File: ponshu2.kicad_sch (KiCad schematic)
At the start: 0 parts

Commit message: create sch file
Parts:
- added U1: STM32F072CBTx, Package_QFP:LQFP-48_7x7mm_P0.5mm, symbol MCU_ST_STM32F0:STM32F072CBTx
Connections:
- new net: U1.23 (VSS), U1.35 (VSS), U1.47 (VSS)
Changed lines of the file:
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@@
 	(generator_version "9.0")
 	(paper "A4")
+	(symbol
+		(lib_id "MCU_ST_STM32F0:STM32F072CBTx")
+		(at 114.3 82.55 0)
+		(unit 1)
+		(exclude_from_sim no)
+		(in_bom yes)
+		(on_board yes)
+		(dnp no)
+		(fields_autoplaced yes)
+		(property "Reference" "U1"
+			(at 118.9833 123.19 0)
+			(effects
+				(font
+					(size 1.27 1.27)
+				)
+				(justify left)
+			)
+		)
+		(property "Value" "STM32F072CBTx"
+			(at 118.9833 125.73 0)
+			(effects
+				(font
+					(size 1.27 1.27)
+				)
+				(justify left)
+			)
+		)
+		(property "Footprint" "Package_QFP:LQFP-48_7x7mm_P0.5mm"
+			(at 99.06 120.65 0)
+			(effects
+				(font
+					(size 1.27 1.27)
+				)
+				(justify right)
+				(hide yes)
+			)
+		)
+		(property "Datasheet" "https://www.st.com/resource/en/datasheet/stm32f072cb.pdf"
+			(at 114.3 82.55 0)
+			(effects
+				(font
+					(size 1.27 1.27)
+				)
+				(hide yes)
+			)
+		)
+		(property "Description" "STMicroelectronics Arm Cortex-M0 MCU, 128KB flash, 16KB RAM, 48 MHz, 2.0-3.6V, 37 GPIO, LQFP48"
+			(at 114.3 82.55 0)
+			(effects
+				(font
+					(size 1.27 1.27)
+				)
+				(hide yes)
+			)
+		)
+		(pin "12"
+		)
+		(pin "13"
+		)
+		(pin "14"
+		)
+		(pin "15"
+		)
+		(pin "16"
+		)
+		(pin "2"
+		)
+		(pin "3"
+		)
+		(pin "4"
+		)
+		(pin "18"
+		)
+		(pin "39"
+		)
+		(pin "40"
+		)
+		(pin "41"
+		)
+		(pin "42"
+		)
+		(pin "43"
+		)
+		(pin "45"
+		)
+		(pin "46"
+		)
+		(pin "21"
+		)
+		(pin "22"
+		)
+		(pin "25"
+		)
+		(pin "26"
+		)
+		(pin "27"
+		)
+		(pin "28"
+		)
+		(pin "1"
+		)
+		(pin "24"
+		)
+		(pin "48"
+		)
+		(pin "23"
+		)
+		(pin "35"
+		)
+		(pin "47"
+		)
+		(pin "9"
+		)
+		(pin "8"
+		)
+		(pin "36"
+		)
+		(pin "5"
+		)
+		(pin "19"
+		)
+		(pin "20"
+		)
+		(pin "10"
+		)
+		(pin "11"
+		)
+		(pin "34"
+		)
+		(pin "37"
+		)
+		(pin "38"
+		)
+		(pin "17"
+		)
+		(pin "29"
+		)
+		(pin "30"
+		)
+		(pin "31"
+		)
+		(pin "32"
+		)
+		(pin "33"
+		)
+		(pin "6"
+		)
+		(pin "44"
+		)
+		(pin "7"
+		)
+		(instances
+			(project ""
+				(path "/9a6ee9bd-87da-4626-8a0a-46205075074e"
+					(reference "U1")
+					(unit 1)
+				)
+			)
+		)
+	)
 	(sheet_instances
 		(path "/"

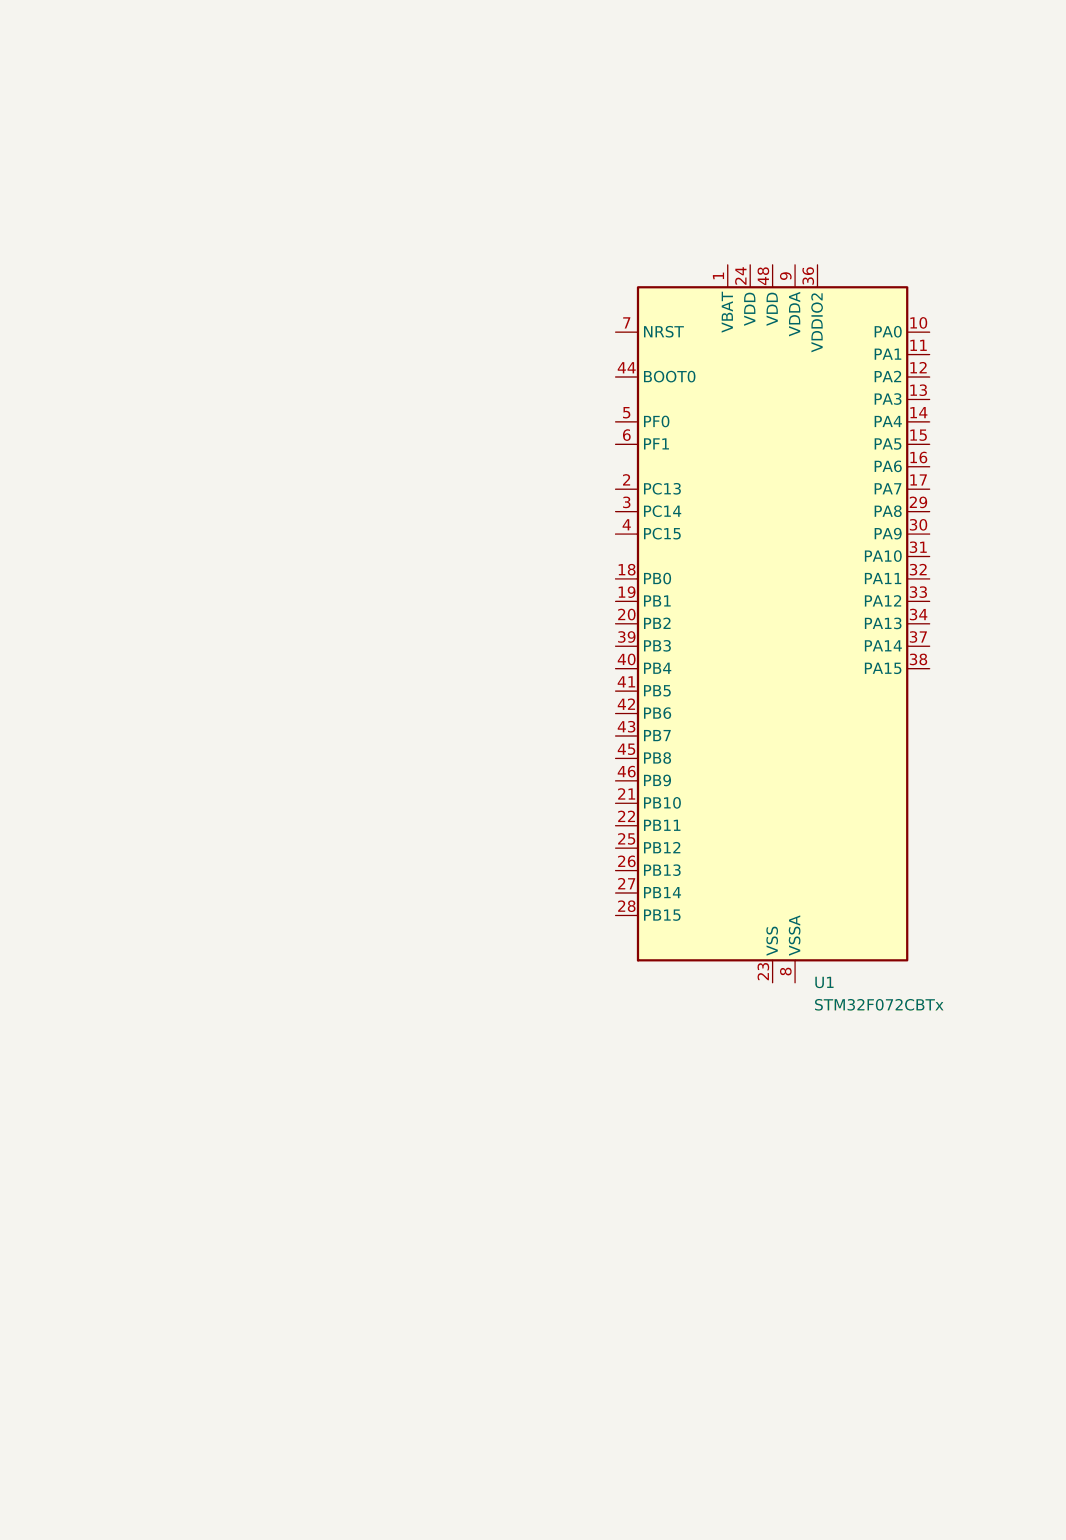
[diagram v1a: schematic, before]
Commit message: chotto PCB tukutayo
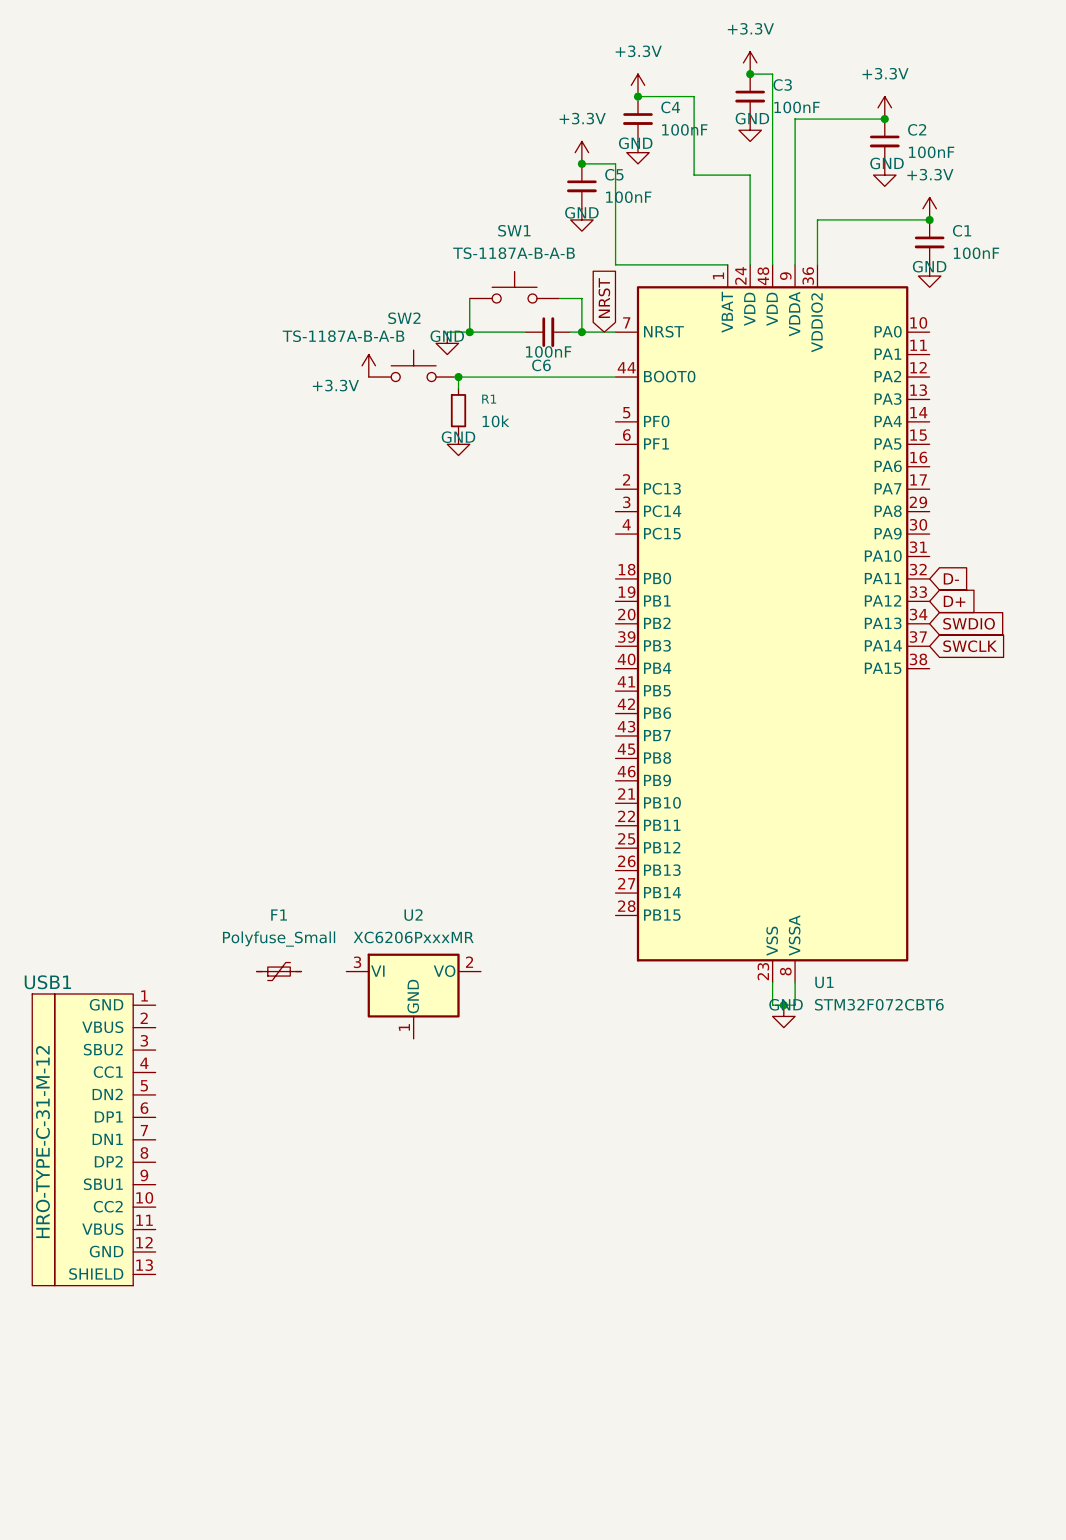
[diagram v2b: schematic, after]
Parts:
- added C1, C2, C3, C4, C5, C6: 100nF, symbol Device:C_Small
- added F1: Polyfuse_Small, symbol Device:Polyfuse_Small
- added R1: 10k, symbol Device:R_Small
- added SW1, SW2: TS-1187A-B-A-B, symbol Switch:SW_Push
- added U2: XC6206PxxxMR, Package_TO_SOT_SMD:SOT-23-3, symbol Regulator_Linear:XC6206PxxxMR
- added USB1: HRO-TYPE-C-31-M-12, symbol Type-C:HRO-TYPE-C-31-M-12
- U1: value STM32F072CBTx -> STM32F072CBT6
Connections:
- net +3.3V: now reaches U1.1 (VBAT)
- net +3.3V: now also U1.24 (VDD), U1.36 (VDDIO2), U1.48 (VDD), U1.9 (VDDA), C1.1, C2.1, C3.1, C4.1, C5.1, SW2.1
- net GND: now reaches U1.23 (VSS), U1.35 (VSS), U1.47 (VSS)
- net GND: now also U1.8 (VSSA), C1.2, C2.2, C3.2, C4.2, C5.2, C6.1, R1.2, SW1.1
- net D-: now reaches U1.32 (PA11)
- net D+: now reaches U1.33 (PA12)
- net SWDIO: now reaches U1.34 (PA13)
- net SWCLK: now reaches U1.37 (PA14)
- net at U1.44 (BOOT0): now also R1.1, SW2.2
- net NRST: now reaches U1.7 (NRST)
- net NRST: now also C6.2, SW1.2

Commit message: PCB daitai owatta kamo
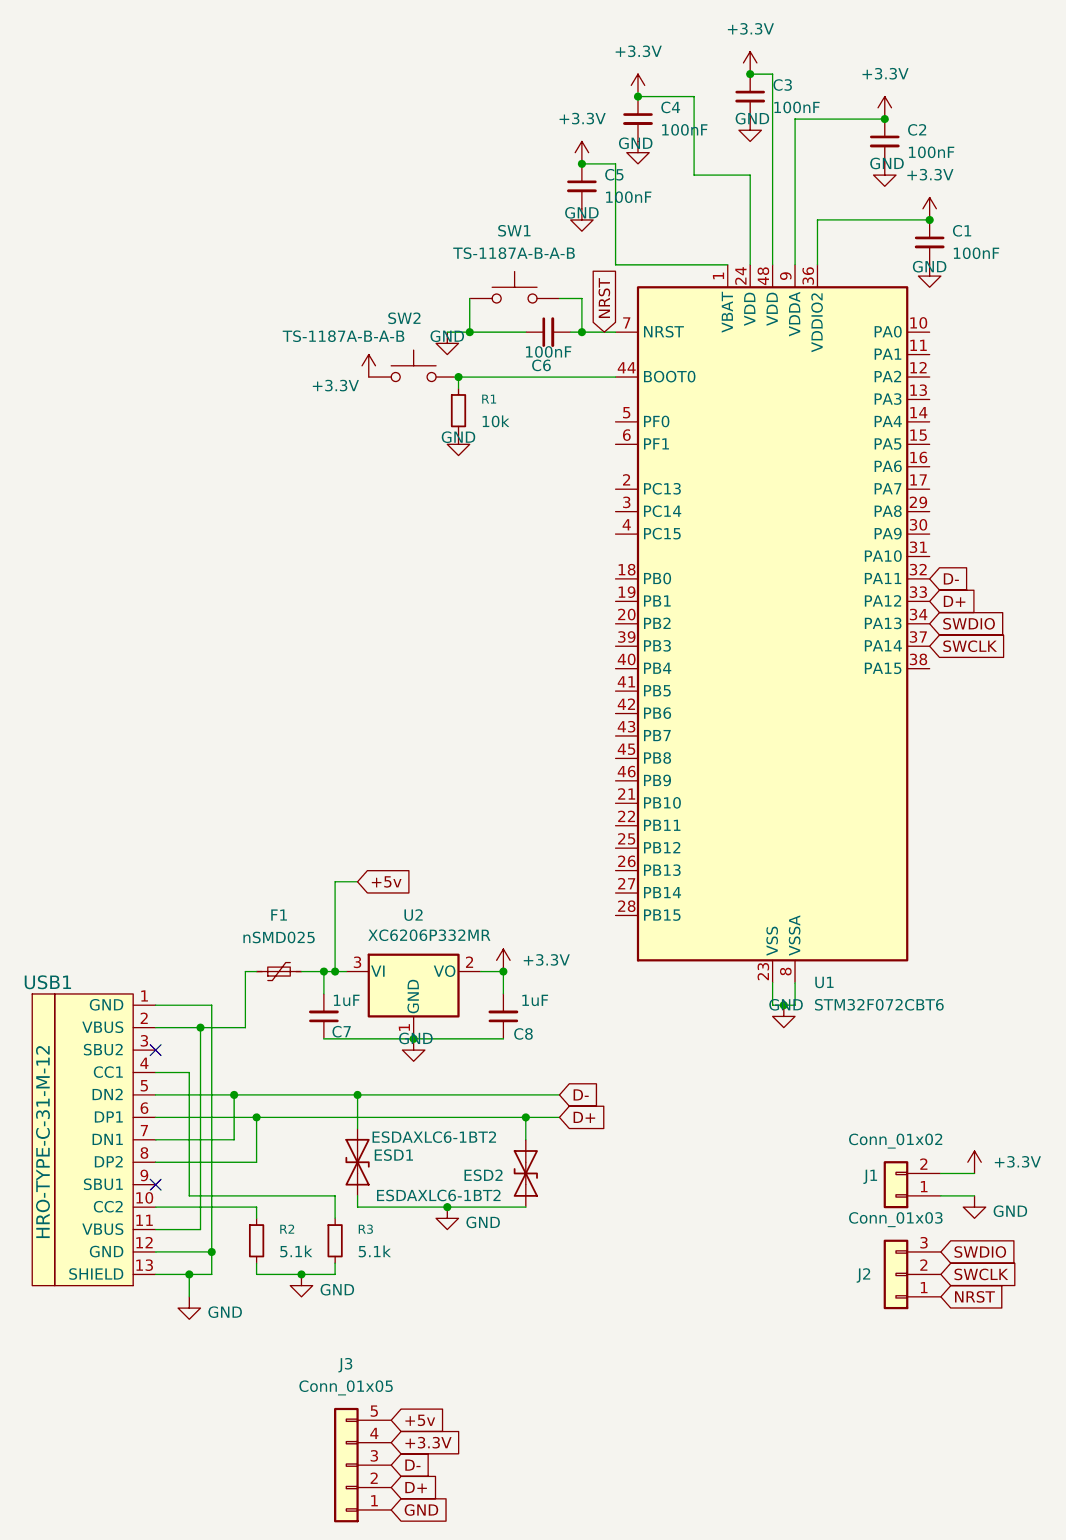
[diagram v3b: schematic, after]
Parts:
- added C7, C8: 1uF, Capacitor_SMD:C_0603_1608Metric, symbol Device:C_Small
- added ESD1, ESD2: ESDAXLC6-1BT2, Diode_SMD:D_SOD-882, symbol Diode:ESD9B3.3ST5G
- added J1: Conn_01x02, Connector_PinHeader_2.54mm:PinHeader_1x02_P2.54mm_Vertical, symbol Connector_Generic:Conn_01x02
- added J2: Conn_01x03, Connector_PinHeader_2.54mm:PinHeader_1x03_P2.54mm_Vertical, symbol Connector_Generic:Conn_01x03
- added J3: Conn_01x05, Connector_PinHeader_2.54mm:PinHeader_1x05_P2.54mm_Vertical, symbol Connector_Generic:Conn_01x05
- added R2, R3: 5.1k, Resistor_SMD:R_0603_1608Metric, symbol Device:R_Small
- C1, C2, C3, C4, C5, C6: footprint (none) -> Capacitor_SMD:C_0402_1005Metric
- F1: value Polyfuse_Small -> nSMD025; footprint (none) -> Fuse:Fuse_1206_3216Metric
- R1: footprint (none) -> Resistor_SMD:R_0603_1608Metric
- SW1, SW2: footprint (none) -> random-keyboard-parts:SKQG-1155865
- U2: value XC6206PxxxMR -> XC6206P332MR
- USB1: footprint (none) -> Connector_USB:USB_C_Receptacle_HRO_TYPE-C-31-M-12
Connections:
- net +3.3V: now also U2.2 (VO), C8.2, J1.2 (Pin_2), J3.4 (Pin_4)
- net D+: now also USB1.6 (DP1), USB1.8 (DP2), ESD2.2 (A2), J3.2 (Pin_2)
- net D-: now also USB1.5 (DN2), USB1.7 (DN1), ESD1.2 (A2), J3.3 (Pin_3)
- net GND: now also U2.1 (GND), USB1.1 (GND), USB1.12 (GND), USB1.13 (SHIELD), C7.1, C8.1, ESD1.1 (A1), ESD2.1 (A1), J1.1 (Pin_1), J3.1 (Pin_1), R2.2, R3.2
- net NRST: now also J2.1 (Pin_1)
- net SWCLK: now also J2.2 (Pin_2)
- net SWDIO: now also J2.3 (Pin_3)
- net at F1.1: now also USB1.11 (VBUS), USB1.2 (VBUS)
- net +5v: now reaches F1.2
- net +5v: now also U2.3 (VI), C7.2, J3.5 (Pin_5)
- net at USB1.10 (CC2): now also R2.1
- net at USB1.4 (CC1): now also R3.1
- no-connect marks 0 -> 2
